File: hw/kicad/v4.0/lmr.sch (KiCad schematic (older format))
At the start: 22 parts

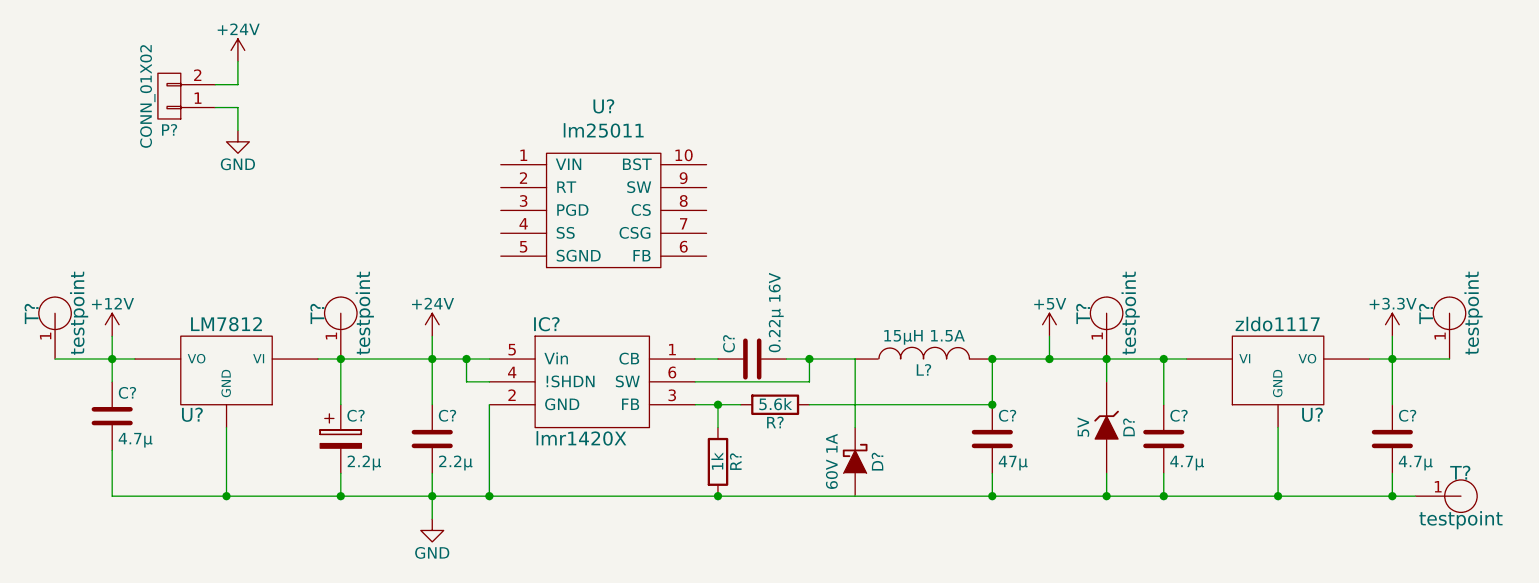
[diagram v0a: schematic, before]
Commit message: v4.0
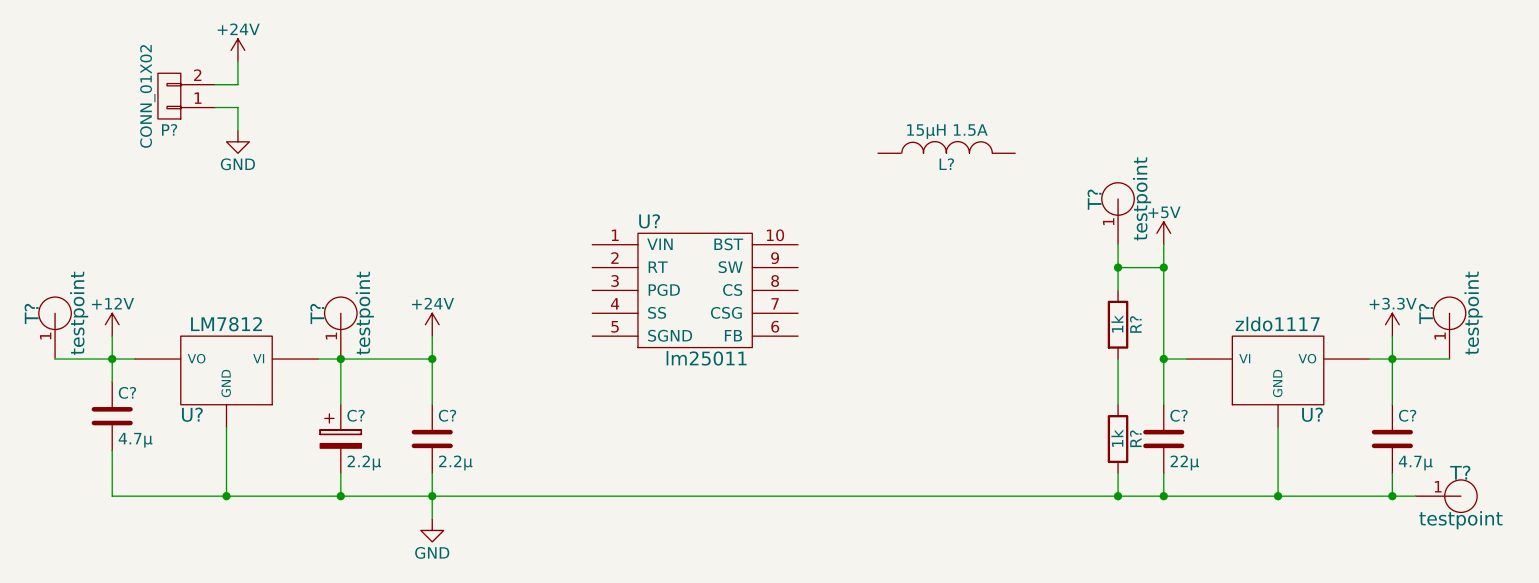
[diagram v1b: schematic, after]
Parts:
- removed C?: 47µ, symbol C
- removed C?: 0.22µ 16V, symbol C
- removed D?: 60V 1A, symbol D_Schottky
- removed D?: 5V, symbol ZENER
- removed IC?: lmr1420X, symbol lmr1420X
- removed R?: 5.6k, symbol R
- removed R?: 1k, symbol R
- removed U?: lm25011, symbol lm25011
- added R? (x2): 1k, symbol R
- added U?: lm25011, symbol lm25011
- C?: value 4.7µ -> 22µ
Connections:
- net +5V: now also R?.1; no longer L?.2
- net GND: now also R?.2
- new net: R?.1, R?.2
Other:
- moved on the sheet: L?, T?
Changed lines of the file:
@@
 $EndDescr
-$Comp
-L lmr1420X IC?
-U 1 1 565A1FC6
-P 4050 3600
-F 0 "IC?" H 3850 3850 60  0000 C CNN
-F 1 "lmr1420X" H 4000 3350 60  0000 C CNN
-F 2 "" H 3950 3600 60  0000 C CNN
-F 3 "" H 3950 3600 60  0000 C CNN
-	1    4050 3600
-	1    0    0    -1
-$EndComp
 $Comp
 L C C?
@@
 $EndComp
 $Comp
-L C C?
-U 1 1 566068C0
-P 5800 3850
-F 0 "C?" H 5825 3950 50  0000 L CNN
-F 1 "47µ" H 5825 3750 50  0000 L CNN
-F 2 "" H 5838 3700 30  0000 C CNN
-F 3 "" H 5800 3850 60  0000 C CNN
-F 4 "6.3V" H 5800 3850 60  0001 C CNN "Voltage"
-	1    5800 3850
-	1    0    0    -1
-$EndComp
-$Comp
-L R R?
-U 1 1 5660690B
-P 4850 3700
-F 0 "R?" V 4930 3700 50  0000 C CNN
-F 1 "5.6k" V 4850 3700 50  0000 C CNN
-F 2 "" V 4780 3700 30  0000 C CNN
-F 3 "" H 4850 3700 30  0000 C CNN
-	1    4850 3700
-	0    1    1    0
-$EndComp
-$Comp
-L R R?
-U 1 1 56606967
-P 4600 3950
-F 0 "R?" V 4680 3950 50  0000 C CNN
-F 1 "1k" V 4600 3950 50  0000 C CNN
-F 2 "" V 4530 3950 30  0000 C CNN
-F 3 "" H 4600 3950 30  0000 C CNN
-	1    4600 3950
-	1    0    0    -1
-$EndComp
-$Comp
-L D_Schottky D?
-U 1 1 566069A3
-P 5200 3950
-F 0 "D?" H 5200 4050 50  0000 C CNN
-F 1 "60V 1A" H 5200 3850 50  0000 C CNN
-F 2 "" H 5200 3950 60  0000 C CNN
-F 3 "" H 5200 3950 60  0000 C CNN
-	1    5200 3950
-	0    1    1    0
-$EndComp
-$Comp
-L C C?
-U 1 1 56606BAA
-P 4750 3500
-F 0 "C?" H 4775 3600 50  0000 L CNN
-F 1 "0.22µ 16V" H 4775 3400 50  0000 L CNN
-F 2 "" H 4788 3350 30  0000 C CNN
-F 3 "" H 4750 3500 60  0000 C CNN
-	1    4750 3500
-	0    -1   -1   0
-$EndComp
-$Comp
 L INDUCTOR L?
 U 1 1 56606C2D
-P 5500 3500
-F 0 "L?" V 5450 3500 50  0000 C CNN
-F 1 "15µH 1.5A" V 5600 3500 50  0000 C CNN
-F 2 "" H 5500 3500 60  0000 C CNN
-F 3 "" H 5500 3500 60  0000 C CNN
-	1    5500 3500
+P 5600 2600
+F 0 "L?" V 5550 2600 50  0000 C CNN
+F 1 "15µH 1.5A" V 5700 2600 50  0000 C CNN
+F 2 "" H 5600 2600 60  0000 C CNN
+F 3 "" H 5600 2600 60  0000 C CNN
+	1    5600 2600
 	0    -1   -1   0
 $EndComp
@@
 P 6550 3850
 F 0 "C?" H 6575 3950 50  0000 L CNN
-F 1 "4.7µ" H 6575 3750 50  0000 L CNN
+F 1 "22µ" H 6575 3750 50  0000 L CNN
 F 2 "" H 6588 3700 30  0000 C CNN
 F 3 "" H 6550 3850 60  0000 C CNN
@@
 $EndComp
 Wire Wire Line
-	4500 3500 4600 3500
-Wire Wire Line
-	4900 3500 5200 3500
-Wire Wire Line
-	5200 3500 5200 3800
-Wire Wire Line
-	5800 3500 5800 3700
-Wire Wire Line
 	1950 4100 7650 4100
 Wire Wire Line
-	5800 3700 5000 3700
-Wire Wire Line
-	5800 4100 5800 4000
-Connection ~ 5800 3700
-Wire Wire Line
-	4700 3700 4500 3700
-Wire Wire Line
-	4600 3800 4600 3700
-Connection ~ 4600 3700
-Wire Wire Line
 	3350 4000 3350 4200
-Connection ~ 4600 4100
-Wire Wire Line
-	3600 3700 3600 4100
-Connection ~ 3600 4100
 Wire Wire Line
 	3350 3400 3350 3700
 Wire Wire Line
-	2850 3500 3600 3500
-Wire Wire Line
-	3600 3600 3500 3600
-Wire Wire Line
-	3500 3600 3500 3500
-Connection ~ 3500 3500
-Wire Wire Line
-	4500 3600 5000 3600
-Wire Wire Line
-	5000 3600 5000 3500
-Connection ~ 5000 3500
-Wire Wire Line
 	7550 4100 7550 4000
-Connection ~ 5800 4100
 Wire Wire Line
 	6550 4000 6550 4100
@@
 Connection ~ 7050 4100
 Wire Wire Line
-	6550 3700 6550 3500
-Wire Wire Line
-	5800 3500 6650 3500
+	6550 3000 6550 3700
 Connection ~ 6550 3500
 Wire Wire Line
@@
 L +5V #PWR?
 U 1 1 5660786F
-P 6050 3400
-F 0 "#PWR?" H 6050 3250 50  0001 C CNN
-F 1 "+5V" H 6050 3540 50  0000 C CNN
-F 2 "" H 6050 3400 60  0000 C CNN
-F 3 "" H 6050 3400 60  0000 C CNN
-	1    6050 3400
+P 6550 3000
+F 0 "#PWR?" H 6550 2850 50  0001 C CNN
+F 1 "+5V" H 6550 3140 50  0000 C CNN
+F 2 "" H 6550 3000 60  0000 C CNN
+F 3 "" H 6550 3000 60  0000 C CNN
+	1    6550 3000
 	1    0    0    -1
 $EndComp
@@
 	1    0    0    -1
 $EndComp
-Connection ~ 5800 3500
 $Comp
 L GND #PWR?
@@
 $EndComp
 Connection ~ 3350 3500
-Wire Wire Line
-	6050 3400 6050 3500
-Connection ~ 6050 3500
 Connection ~ 7550 3500
 $Comp
@@
 	2500 2400 2500 2500
 $Comp
-L ZENER D?
-U 1 1 56694BC4
-P 6300 3800
-F 0 "D?" H 6300 3900 50  0000 C CNN
-F 1 "5V" H 6300 3700 50  0000 C CNN
-F 2 "" H 6300 3800 60  0000 C CNN
-F 3 "" H 6300 3800 60  0000 C CNN
-	1    6300 3800
-	0    1    1    0
-$EndComp
-Wire Wire Line
-	6300 3600 6300 3500
-Connection ~ 6300 3500
-Wire Wire Line
-	6300 4000 6300 4100
-Connection ~ 6300 4100
-$Comp
 L CONN_01X02 P?
 U 1 1 566CDEAC
@@
 L testpoint T?
 U 1 1 56819741
-P 6300 3300
-F 0 "T?" H 6300 3400 60  0000 C CNN
-F 1 "testpoint" H 6300 3200 60  0000 C CNN
-F 2 "" H 6300 3300 60  0000 C CNN
-F 3 "" H 6300 3300 60  0000 C CNN
-	1    6300 3300
+P 6350 2800
+F 0 "T?" H 6350 2900 60  0000 C CNN
+F 1 "testpoint" H 6350 2700 60  0000 C CNN
+F 2 "" H 6350 2800 60  0000 C CNN
+F 3 "" H 6350 2800 60  0000 C CNN
+	1    6350 2800
 	0    -1   -1   0
 $EndComp
@@
 	1    0    0    -1
 $EndComp
+Wire Wire Line
+	2850 3500 3350 3500
+$Comp
+L R R?
+U 1 1 571088D2
+P 6350 3850
+F 0 "R?" V 6430 3850 50  0000 C CNN
+F 1 "1k" V 6350 3850 50  0000 C CNN
+F 2 "" V 6280 3850 30  0000 C CNN
+F 3 "" H 6350 3850 30  0000 C CNN
+	1    6350 3850
+	1    0    0    -1
+$EndComp
 $Comp
 L lm25011 U?
-U 1 1 570D946D
-P 4100 2850
-F 0 "U?" H 4100 3303 60  0000 C CNN
-F 1 "lm25011" H 4100 3197 60  0000 C CNN
-F 2 "" H 4100 2850 60  0000 C CNN
-F 3 "" H 4100 2850 60  0000 C CNN
-	1    4100 2850
-	1    0    0    -1
-$EndComp
+U 1 1 57108924
+P 4500 3200
+F 0 "U?" H 4300 3500 60  0000 C CNN
+F 1 "lm25011" H 4550 2900 60  0000 C CNN
+F 2 "" H 4500 3200 60  0000 C CNN
+F 3 "" H 4500 3200 60  0000 C CNN
+	1    4500 3200
+	1    0    0    -1
+$EndComp
+$Comp
+L R R?
+U 1 1 571089CF
+P 6350 3350
+F 0 "R?" V 6430 3350 50  0000 C CNN
+F 1 "1k" V 6350 3350 50  0000 C CNN
+F 2 "" V 6280 3350 30  0000 C CNN
+F 3 "" H 6350 3350 30  0000 C CNN
+	1    6350 3350
+	1    0    0    -1
+$EndComp
+Wire Wire Line
+	6550 3500 6650 3500
+Wire Wire Line
+	6350 3000 6350 3200
+Wire Wire Line
+	6350 3100 6550 3100
+Connection ~ 6550 3100
+Connection ~ 6350 3100
+Wire Wire Line
+	6350 3500 6350 3700
+Wire Wire Line
+	6350 4000 6350 4100
+Connection ~ 6350 4100
 $EndSCHEMATC
